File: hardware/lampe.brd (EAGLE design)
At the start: 63.2 x 62.2 mm, 45 parts, among them IC1 LM393N, IC2 ATMEGA168-20P, IC3 DS1307, Q1 IRFU9024N, Q2 16MHz, Q3 32.768kHz, T1 BC457B, T2 BC557B, T3 BC457B

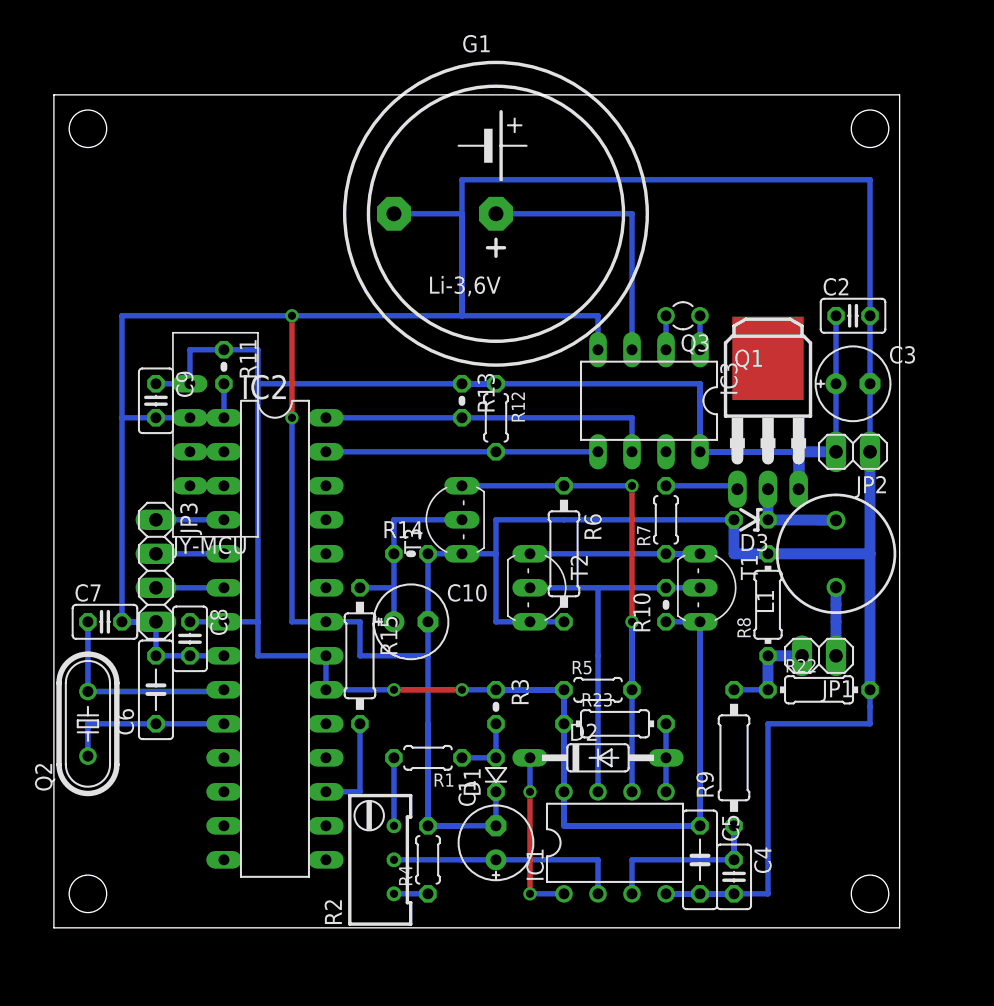
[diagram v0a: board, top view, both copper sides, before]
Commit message: Cleanup
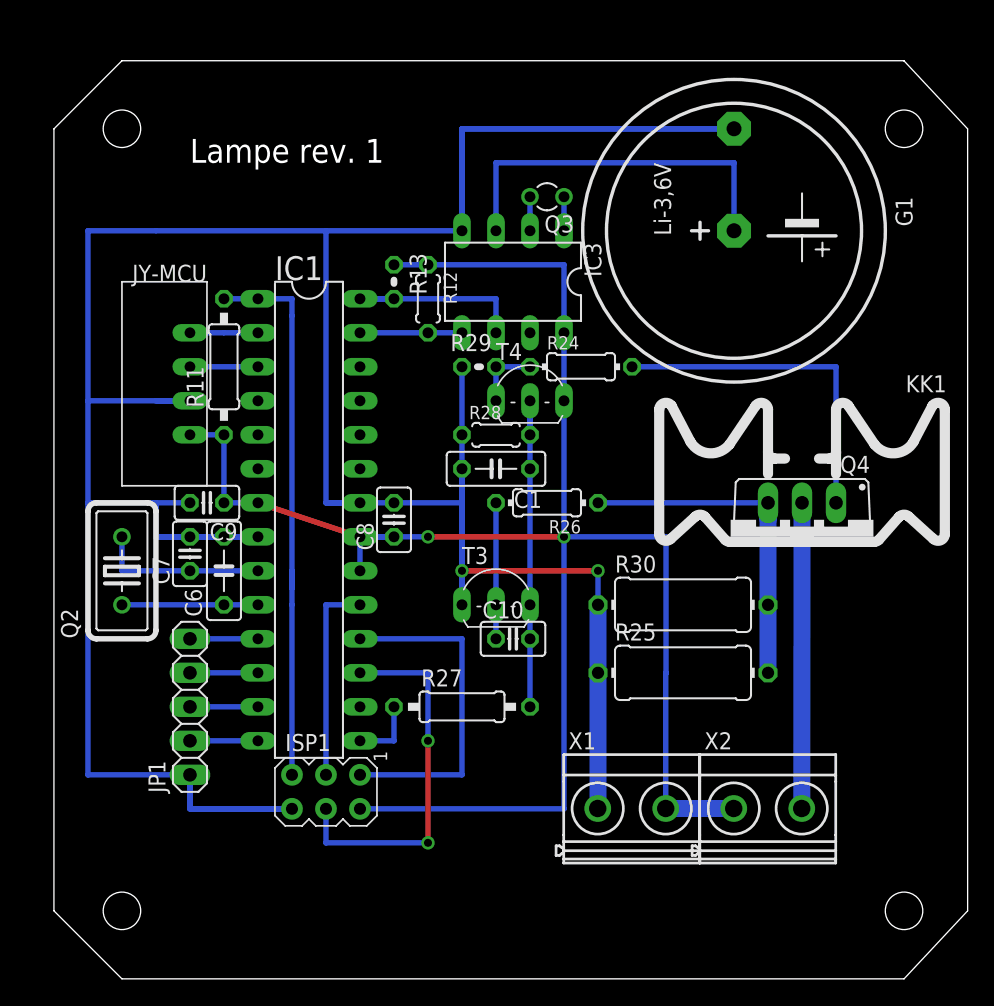
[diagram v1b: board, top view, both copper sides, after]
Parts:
- removed C2: 100nF, rcl:C025-025X050
- removed C3: 100uF, rcl:E2,5-6E
- removed C4: 22pF, rcl:C025-025X050
- removed C5: 100nF, rcl:C050-025X075
- removed D1: 1N4148, diode:D-2.5
- removed D2: 1N4148, diode:DO35-10
- removed D3: SB140, diode:ZDIO-2.5
- removed IC2: ATMEGA168-20P, adafruit:DIL28-3
- removed JP2: SUPPLY, pinhead:1X02
- removed JP3: (no value), pinhead:1X04
- removed L1: 100uH, rcl:6000-XXXX-RC
- removed Q1: IRFU9024N, transistor-power:I-PAK_TO251AA
- removed R1, R5: 10k, rcl:0204/5
- removed R10, R3: 4.7k, rcl:0204V
- removed R14: 10k, rcl:0204V
- removed R15: 15k, rcl:0207/10
- removed R2: 10k, rcl:RTRIM64W
- removed R22, R8: 1R*, rcl:0204/7
- removed R23: 4.7k, rcl:0204/7
- removed R4: 1k, rcl:0204/5
- removed R6: 10k, rcl:0207/10
- removed R7: 10R, rcl:0204/5
- removed R9: 1k, rcl:0207/10
- removed T1: BC457B, transistor:TO92-EBC
- removed T2: BC557B, transistor:TO92-EBC
- added ISP1: AVRISP-6, adafruit:AVRISP
- added KK1: PF750, heatsink:PF752
- added Q4: BUZ11BV, transistor-power:TO220BV
- added R24: 10, rcl:0204/7
- added R25, R30: 1W, rcl:0411/12
- added R26: 560, rcl:0204/7
- added R27: 10k, rcl:0207/10
- added R28: 10k, rcl:0204/5
- added R29: 1k, rcl:0204V
- added T4: BC547B, transistor-neu-to92:TO92-EBC
- added X1, X2: MKDSN1,5/2-5,08, con-phoenix-508:MKDSN1,5/2-5,08
- C1: value 1uF -> 100nF; device rcl:E2,5-6E -> rcl:C050-025X075
- C10: value 10uF -> 100pF; device rcl:E2,5-6E -> rcl:C025-025X050
- IC1: value LM393N -> ATMEGA168-20P; device linear:DIL08 -> adafruit:DIL28-3
- JP1: value LED -> GPIO; device pinhead:1X02 -> pinhead:1X05
- Q2: value 16MHz -> 16Mhz; device crystal:HC49/S -> adafruit:HC18U-V
- R11: device rcl:0204V -> rcl:0207/10
- T3: value BC457B -> BC547B; device transistor:TO92-EBC -> transistor-neu-to92:TO92-EBC
- moved JP1 47.1 mm to (40.6, 31.8), turned to 90 degrees
- moved IC1 33.2 mm to (49.5, 45.7), turned to 270 degrees
- moved C1 27.9 mm to (63.5, 49.5), turned to 180 degrees
- moved G1 17.8 mm to (81.3, 67.3), turned to 270 degrees
- moved C8 17.6 mm to (55.9, 45.7), turned to 90 degrees
- moved IC3 13.5 mm to (64.8, 63.5)
- moved Q3 13.5 mm to (67.3, 69.8)
- moved Q2 11.7 mm to (35.6, 41.9)
- moved R13 10.2 mm to (55.9, 63.5)
- moved C6 10.2 mm to (43.2, 41.9)
- moved R12 10.2 mm to (58.4, 62.2)
- moved C9 8.52 mm to (41.9, 47.0), turned to 180 degrees
- moved C7 8.13 mm to (40.6, 43.2), turned to 90 degrees
- moved C10 7.73 mm to (64.8, 36.8)
- moved T3 6.35 mm to (63.5, 40.6), turned to 0 degrees
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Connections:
- removed net N$10: IC1.7, R10.2, T1.B, T2.B
- removed net N$11: R7.1, T1.E, T2.E
- removed net N$15: D3.C, L1.2, Q1.2
- removed net N$16: Q1.1, R7.2
- removed net N$17: JP1.1, L1.1
- removed net N$20: IC2.1, R11.2
- removed net N$25: IC2.17, R15.2
- removed net N$26: C10.+, R14.1, R15.1, T3.B
- removed net N$27: IC2.5, JP3.2
- removed net N$28: IC2.6, JP3.3
- removed net N$30: C7.1, IC2.9, Q2.2
- new net N$37: Q4.G, R24.2
- new net N$38: Q4.D, X2.2
- new net N$39: Q4.S, R25.2, R26.1, R30.2
- new net N$40: C10.1, R26.2, T3.B
- new net N$41: C1.1, C10.2, R27.2, R28.2, T3.C, T4.B
- new net N$43: R24.1, R29.2, T4.E
- net +5V: now also IC1.20, IC1.21, IC1.7, ISP1.2, T4.C, X1.2, X2.1; no longer C2.1, C3.+, C5.1, IC1.8, IC2.20, IC2.21, IC2.7, JP2.2, Q1.3, R10.1, R23.1, R3.1, R5.1, T1.C
- net GND: now also C1.2, IC1.22, IC1.8, ISP1.6, JP1.1, R25.1, R28.1, R29.1, R30.1, X1.1; no longer C1.-, C10.-, C2.2, C3.-, C4.2, C5.2, D1.C, D3.A, IC1.4, IC2.22, IC2.8, JP2.1, JP3.4, R14.2, R22.2, R4.2, R6.2, R8.2, T2.C
- net N$1: now also IC1.15, R27.1; no longer D1.A, R1.1, R3.2
- net N$12: now also C7.1, IC1.9, Q2.2; no longer IC2.3, U$1.RXD
- net N$18: now also IC1.10; no longer IC2.10
- net N$19: now also IC1.28; no longer IC2.28
- net N$2: now also IC1.18, ISP1.1; no longer R1.2, R2.3
- net N$21: now also IC1.27; no longer IC2.27
- net N$23: now also IC1.3; no longer IC2.2
- net N$24: now also IC1.2, U$1.RXD; no longer IC2.4, JP3.1
- net N$3: now also IC1.19, ISP1.3; no longer C1.+, IC1.2, R2.2
- net N$4: now also IC1.1, ISP1.5, R11.2; no longer R2.1, R4.1
- net N$5: now also IC1.17, ISP1.4; no longer JP1.2, R22.1, R8.1, R9.2
- net N$6: now also IC1.12, JP1.4; no longer C4.1, IC1.3, R9.1
- net N$7: now also IC1.11, JP1.5; no longer D2.C, IC1.1
- net N$8: now also IC1.13, JP1.3; no longer D2.A, IC1.5, R23.2
- net N$9: now also IC1.14, JP1.2; no longer IC1.6, R5.2, R6.1, T3.C
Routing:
- net +5V: track 229.9 -> 140.2 mm
- net N$4: track 2.54 -> 43.2 mm
- net GND: track 336.6 -> 298.5 mm
- net N$9: track 40.6 -> 5.08 mm, vias 2 -> 0
- net N$10: track 27.9 -> 0.00 mm
- net N$39: track 0.00 -> 26.7 mm
- net N$37: track 0.00 -> 25.4 mm
- net N$41: track 0.00 -> 25.4 mm
- net N$5: track 7.62 -> 31.8 mm, vias 0 -> 2
- net N$38: track 0.00 -> 22.8 mm
- net N$2: track 5.08 -> 25.4 mm
- net N$30: track 15.5 -> 0.00 mm
- net N$26: track 15.2 -> 0.00 mm
- net N$11: track 15.2 -> 0.00 mm
- net N$21: track 20.3 -> 7.62 mm
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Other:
- board size 63.2 x 62.2 mm -> 68.2 x 68.6 mm
- board text added: "Lampe rev. 1"
